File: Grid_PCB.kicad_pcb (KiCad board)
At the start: 2 copper layers, 223.2 x 22 mm, 41 parts, among them J1 Conn_01x04_Female, J10 LED_Conn, J11 Power_Conn, J2 Conn_01x04_Female, J3 Conn_01x04_Female, J4 Conn_01x04_Female, J5 Conn_01x04_Female, J6 Conn_01x04_Female, J7 Conn_01x04_Female, J8 Conn_01x04_Female, J9 ESP_Conn, U1 SN74HC151N

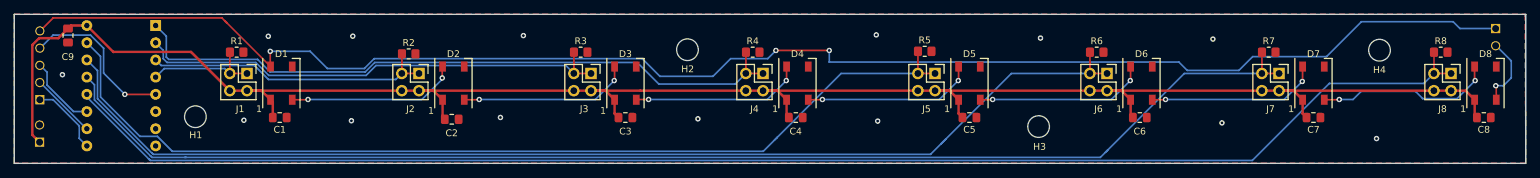
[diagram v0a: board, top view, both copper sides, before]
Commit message: first attempt at waves
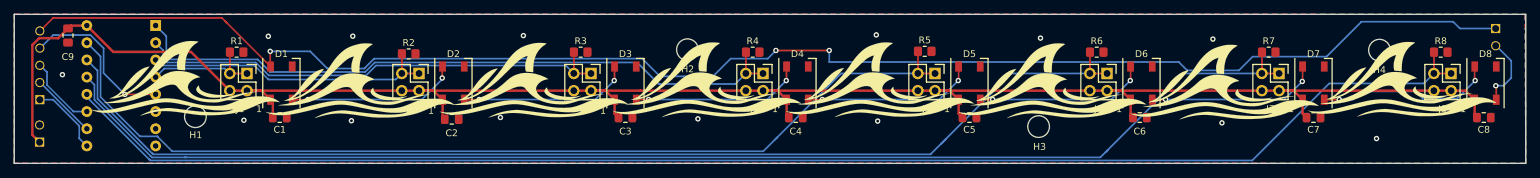
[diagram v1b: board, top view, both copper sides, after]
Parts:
- added G***: LOGO, grid:Wave, F.Cu at (68.3, 92.9)
- added G***: LOGO, grid:Wave, F.Cu at (248.0, 93.0)
- added G***: LOGO, grid:Wave, F.Cu at (221.7, 93.4)
- added G***: LOGO, grid:Wave, F.Cu at (196.3, 93.2)
- added G***: LOGO, grid:Wave, F.Cu at (170.9, 93.1)
- added G***: LOGO, grid:Wave, F.Cu at (145.3, 93.1)
- added G***: LOGO, grid:Wave, F.Cu at (119.7, 93.2)
- added G***: LOGO, grid:Wave, F.Cu at (94.1, 93.2)

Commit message: wave pattern attempt
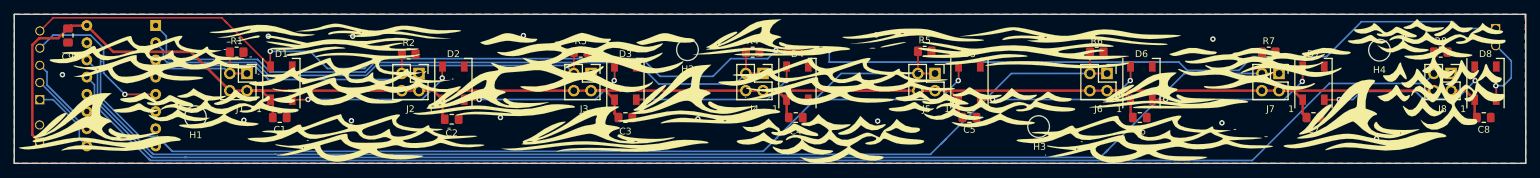
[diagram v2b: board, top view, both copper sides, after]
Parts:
- removed the G*** at (68.3, 92.9)
- removed the G*** at (248.0, 93.0)
- removed the G*** at (221.7, 93.4)
- removed the G*** at (196.3, 93.2)
- removed the G*** at (170.9, 93.1)
- removed the G*** at (145.3, 93.1)
- removed the G*** at (119.7, 93.2)
- removed the G*** at (94.1, 93.2)
- added G***: LOGO, grid:wave_pattern, F.Cu at (153.9, 95.1)

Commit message: wave 2
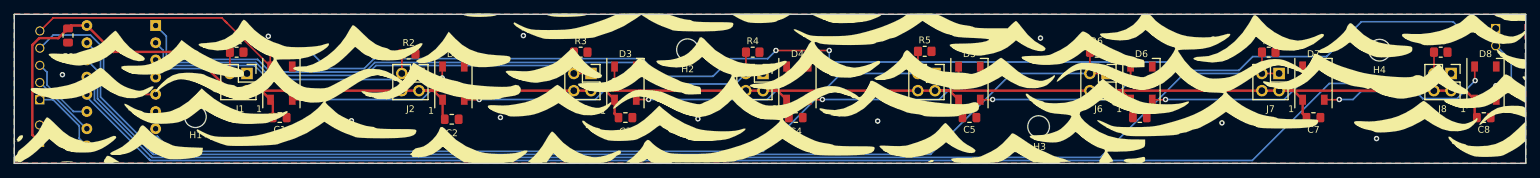
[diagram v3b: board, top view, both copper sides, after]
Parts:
- removed the G*** at (153.9, 95.1)
- added G***: LOGO, grid:wave_pattern_2_light, F.Cu at (154.1, 95.1)
- added G***: LOGO, grid:wave_pattern_2, F.Cu at (154.9, 94.6)

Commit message: wave 2 light
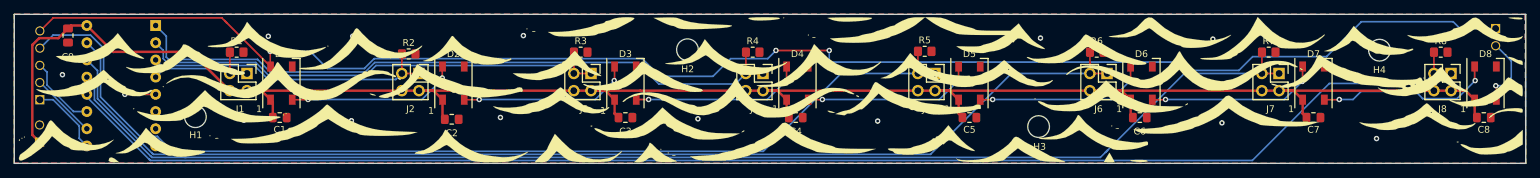
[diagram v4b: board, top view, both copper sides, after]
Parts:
- removed the G*** at (154.9, 94.6)
- moved G*** 0.72 mm to (154.8, 94.9)

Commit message: wave 3
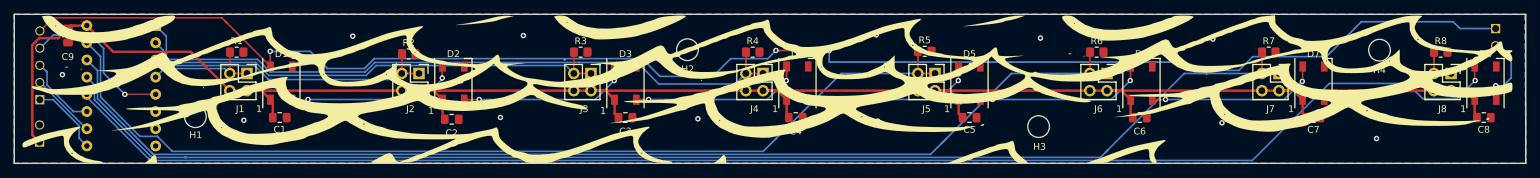
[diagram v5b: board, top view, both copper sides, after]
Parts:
- removed the G*** at (154.8, 94.9)
- added G***: LOGO, grid:wave_pattern_3, F.Cu at (154.3, 94.9)
